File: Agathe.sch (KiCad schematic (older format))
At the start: 161 parts, among them U1 Elite-C

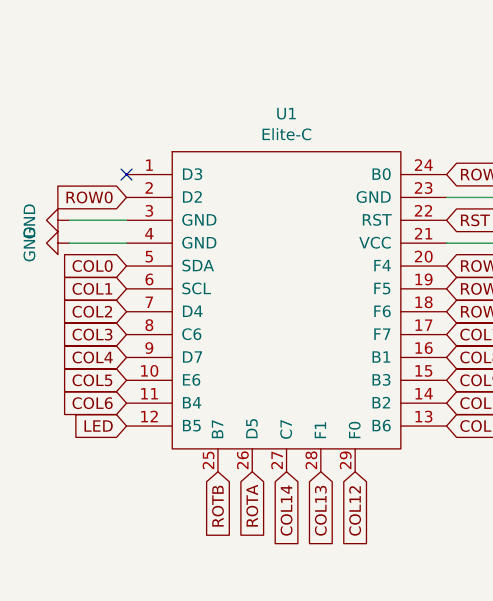
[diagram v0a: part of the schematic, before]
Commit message: elite-c horizontal
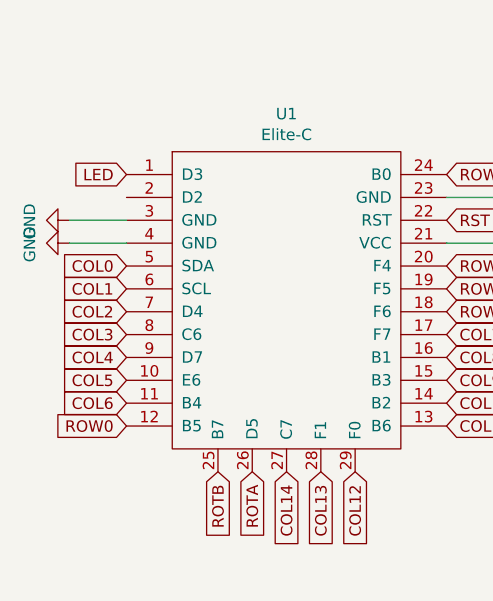
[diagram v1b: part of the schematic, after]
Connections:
- net LED: now also U1.1 (D3); no longer U1.12 (B5)
- net ROW0: now also U1.12 (B5); no longer U1.2 (D2)
- no-connect marks 2 -> 1
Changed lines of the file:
@@
 	1    0    0    -1
 $EndComp
-Text GLabel 1300 1450 0    50   Input ~ 0
+Text GLabel 1300 2450 0    50   Input ~ 0
 ROW0
 Text GLabel 2700 1350 2    50   Input ~ 0
@@
 Text GLabel 2000 2650 3    50   Input ~ 0
 COL14
-Text GLabel 1300 2450 0    50   Input ~ 0
+Text GLabel 1300 1350 0    50   Input ~ 0
 LED
 Text GLabel 1700 2650 3    50   Input ~ 0
@@
 Text GLabel 2700 1550 2    50   Input ~ 0
 RST
-NoConn ~ 1300 1350
 $EndSCHEMATC
